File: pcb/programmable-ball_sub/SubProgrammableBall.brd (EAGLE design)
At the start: 20.5 x 20 mm, 9 parts, among them CON1 B4B-ZR-SM4-TF, U2 LSM6DS0TR

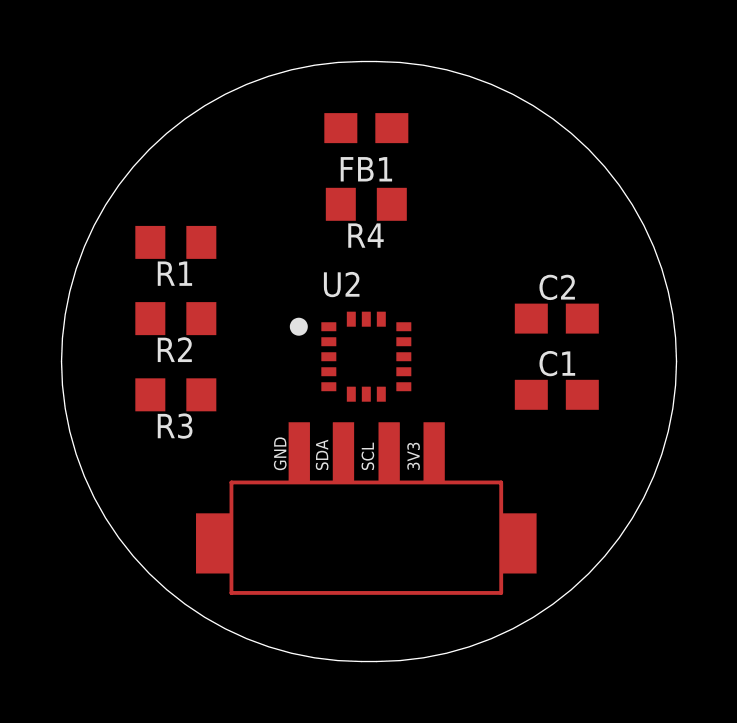
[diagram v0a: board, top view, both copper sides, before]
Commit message: brd, schの更新
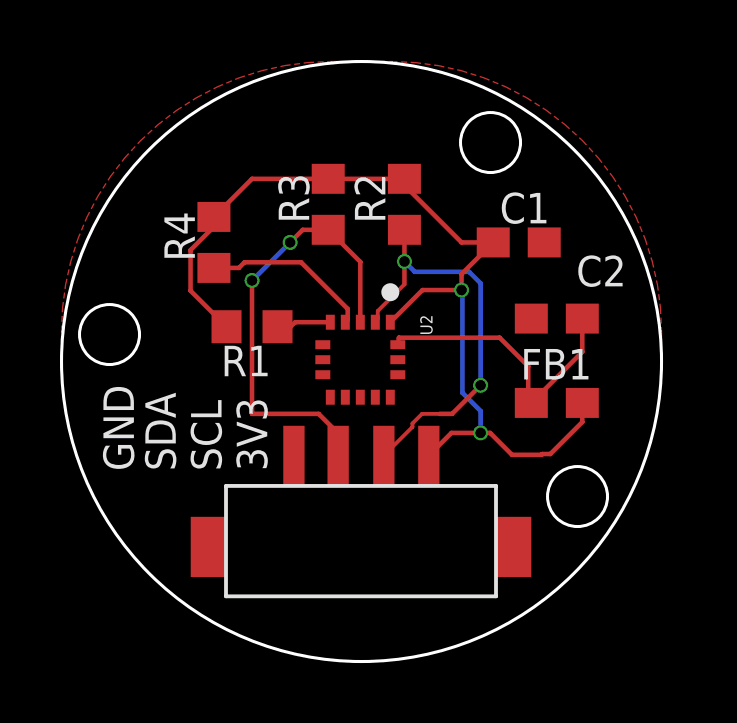
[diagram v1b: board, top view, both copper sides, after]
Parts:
- moved FB1 11.1 mm to (16.5, 8.62), turned to 180 degrees
- moved R2 8.52 mm to (11.4, 15.2), turned to 90 degrees
- moved R3 8.13 mm to (8.89, 15.2), turned to 90 degrees
- moved C1 5.24 mm to (15.2, 14.0)
- moved R4 5.24 mm to (5.08, 14.0), turned to 90 degrees
- moved R1 3.79 mm to (6.35, 11.2)
- moved U2 0.22 mm to (9.96, 10.1), turned to 270 degrees
- moved CON1 0.21 mm to (9.98, 5.34)
- turned C2 to 180 degrees
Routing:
- net +3V3: track 0.00 -> 32.0 mm, vias 0 -> 2
- net N$3: track 0.00 -> 15.1 mm, vias 0 -> 2
- net SCL: track 0.00 -> 14.0 mm, vias 0 -> 2
- net N$1: track 0.00 -> 9.78 mm
- net N$5: track 0.00 -> 5.66 mm
- net N$2: track 0.00 -> 1.82 mm
- added copper zone on layer 1, net GND
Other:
- board size 20.5 x 20 mm -> 20 x 20 mm
